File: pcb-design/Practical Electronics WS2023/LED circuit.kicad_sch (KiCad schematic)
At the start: 16 parts

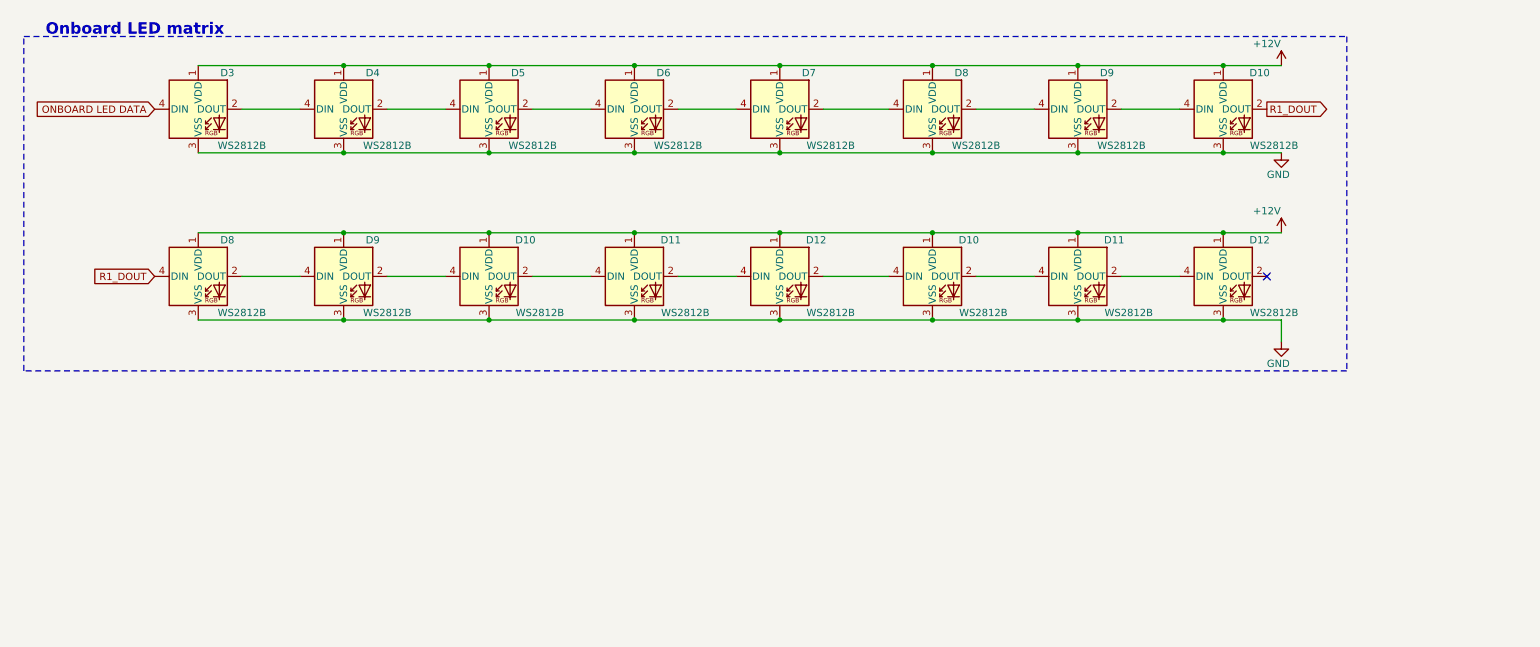
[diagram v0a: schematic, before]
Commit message: Update schematic
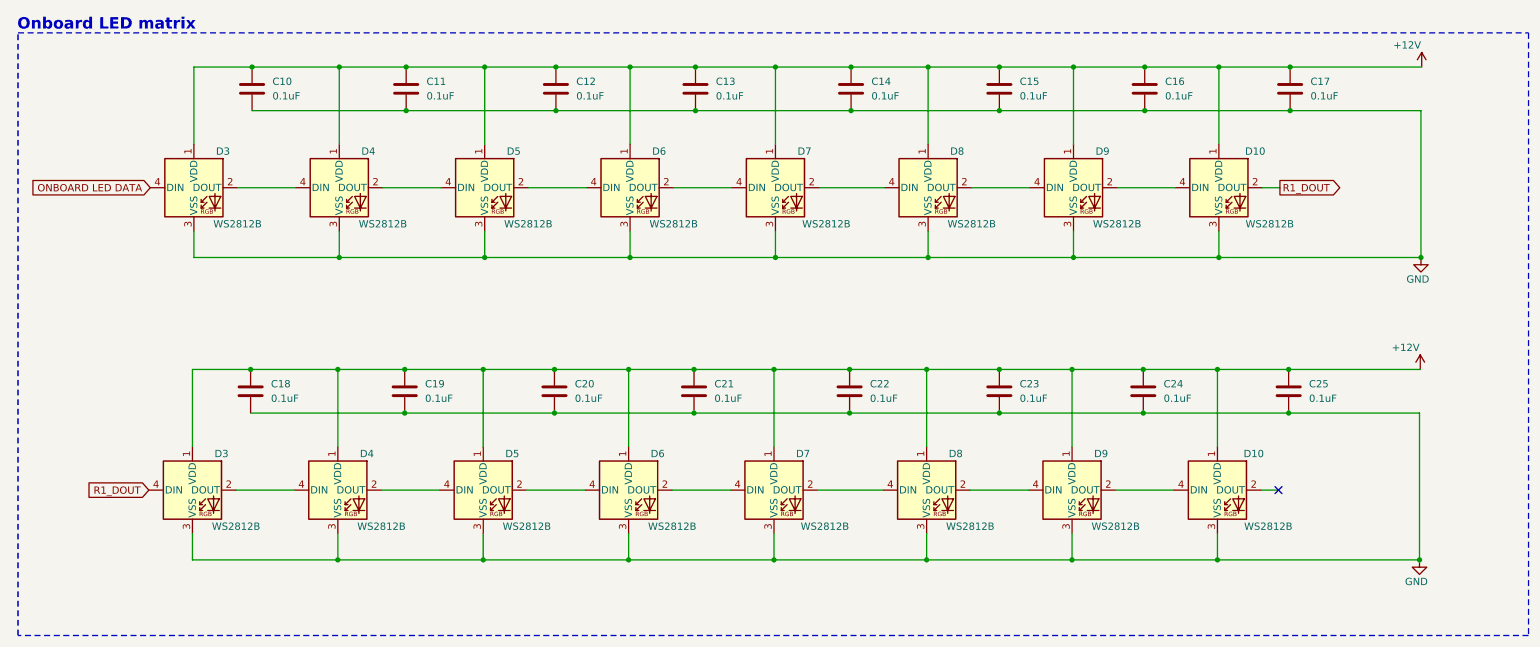
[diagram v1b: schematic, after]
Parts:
- removed D10 (x2), D11 (x2), D12 (x2): WS2812B, LED_SMD:LED_WS2812B_PLCC4_5.0x5.0mm_P3.2mm, symbol LED:WS2812B
- added C10, C11, C12, C13, C14, C15, C16, C17, C18, C19, C20, C21, C22, C23, C24, C25: 0.1uF, symbol Device:C
- added D10, D3, D4, D5, D6, D7: WS2812B, LED_SMD:LED_WS2812B_PLCC4_5.0x5.0mm_P3.2mm, symbol LED:WS2812B
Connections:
- net +12V: now also C10.1, C11.1, C12.1, C13.1, C14.1, C15.1, C16.1, C17.1, C18.1, C19.1, C20.1, C21.1, C22.1, C23.1, C24.1, C25.1, D10.1 (VDD), D3.1 (VDD), D4.1 (VDD), D5.1 (VDD), D6.1 (VDD), D7.1 (VDD)
- net GND: now also C10.2, C11.2, C12.2, C13.2, C14.2, C15.2, C16.2, C17.2, C18.2, C19.2, C20.2, C21.2, C22.2, C23.2, C24.2, C25.2, D10.3 (VSS), D3.3 (VSS), D4.3 (VSS), D5.3 (VSS), D6.3 (VSS), D7.3 (VSS)
- net R1_DOUT: now also D3.4 (DIN); no longer D8.4 (DIN)
- net at D9.2 (DOUT): now also D10.4 (DIN)
- new net: D7.2 (DOUT), D8.4 (DIN)
- new net: D5.2 (DOUT), D6.4 (DIN)
- new net: D4.2 (DOUT), D5.4 (DIN)
- new net: D6.2 (DOUT), D7.4 (DIN)
- new net: D3.2 (DOUT), D4.4 (DIN)
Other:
- moved on the sheet: D10, D3, D4, D5, D6, D7, D8, D9
